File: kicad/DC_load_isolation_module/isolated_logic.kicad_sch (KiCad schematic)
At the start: 40 parts, among them Q17 MMBT5401, Q18 MMBT5401, Q2 MMBT5401, Q3 MMBT5401, Q4 MMBT5551L, Q7 MMBT5551L, U1 LTV-817S, U3 LTV-817S

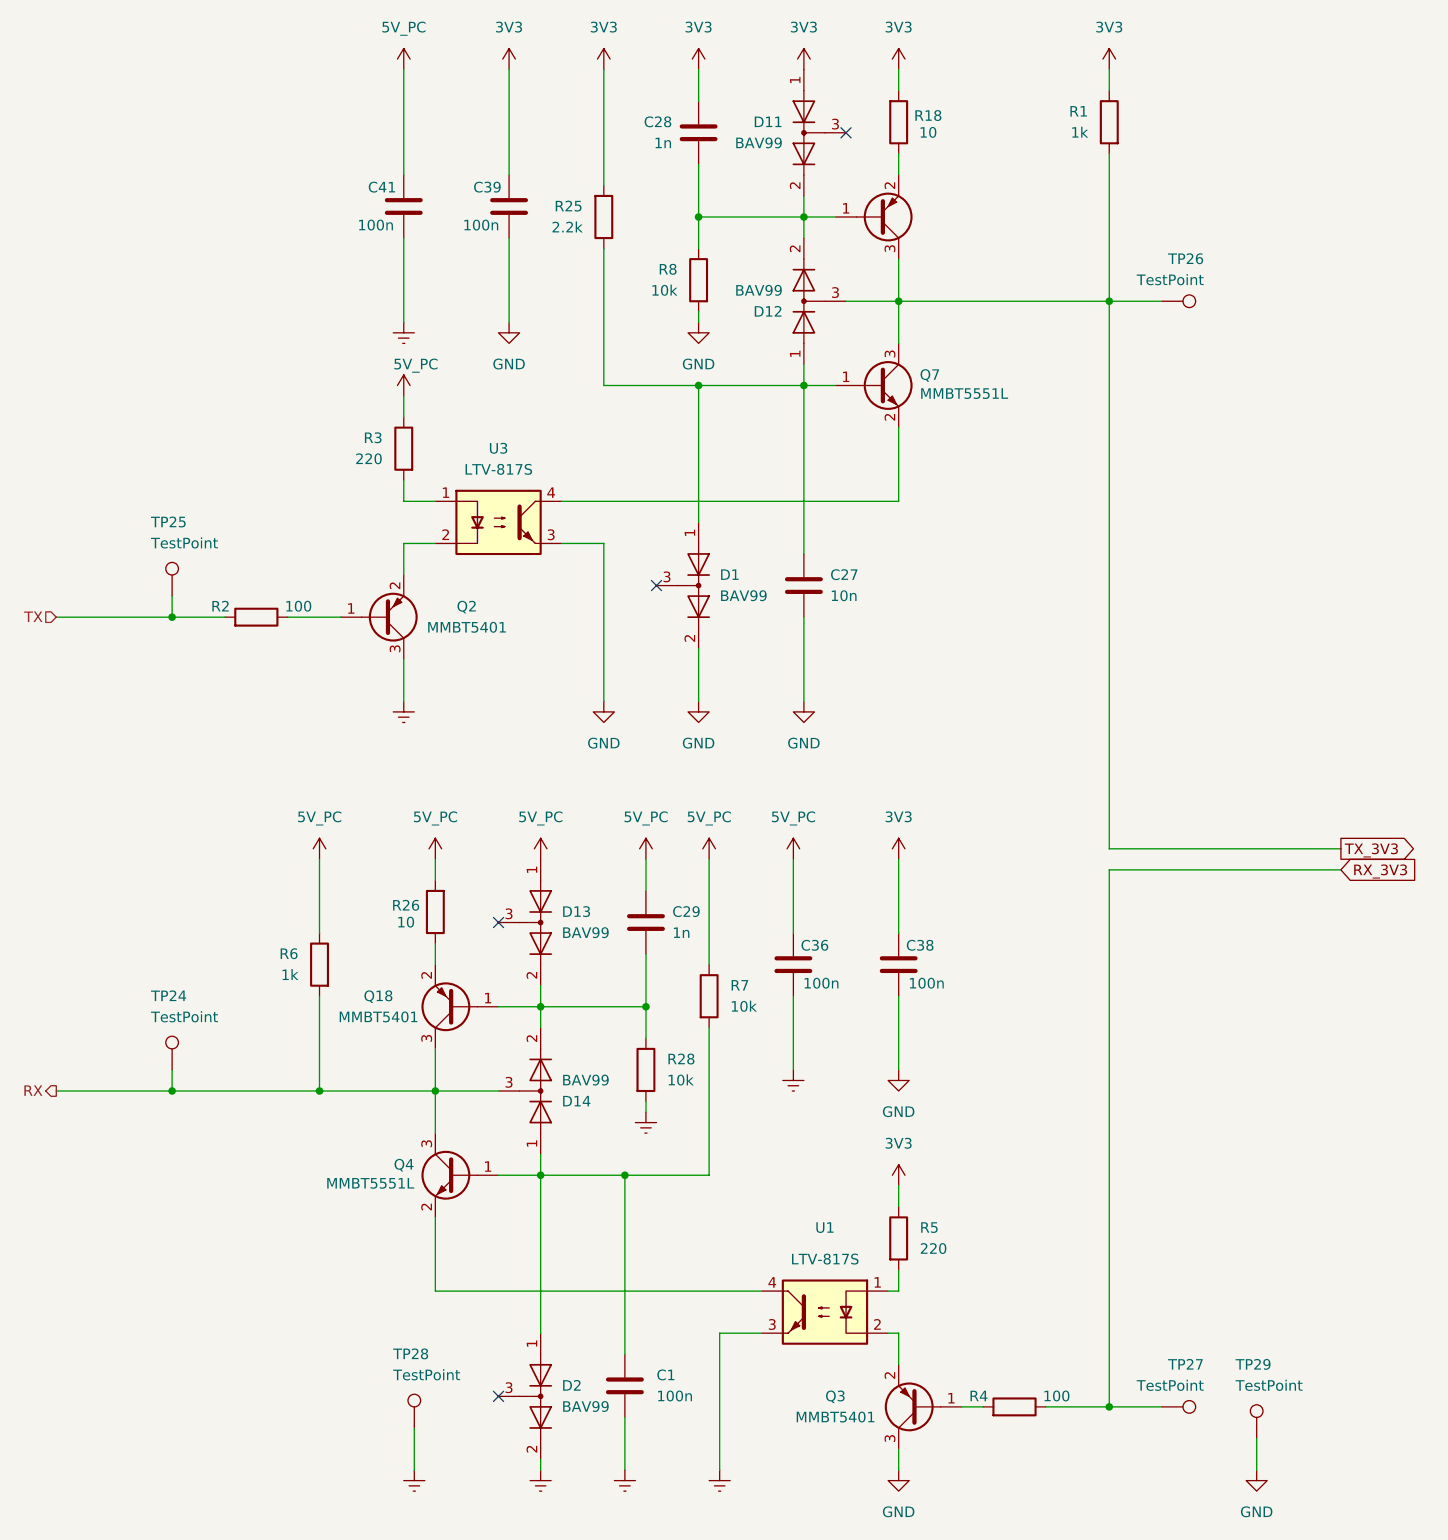
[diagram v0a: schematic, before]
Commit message: Fixes
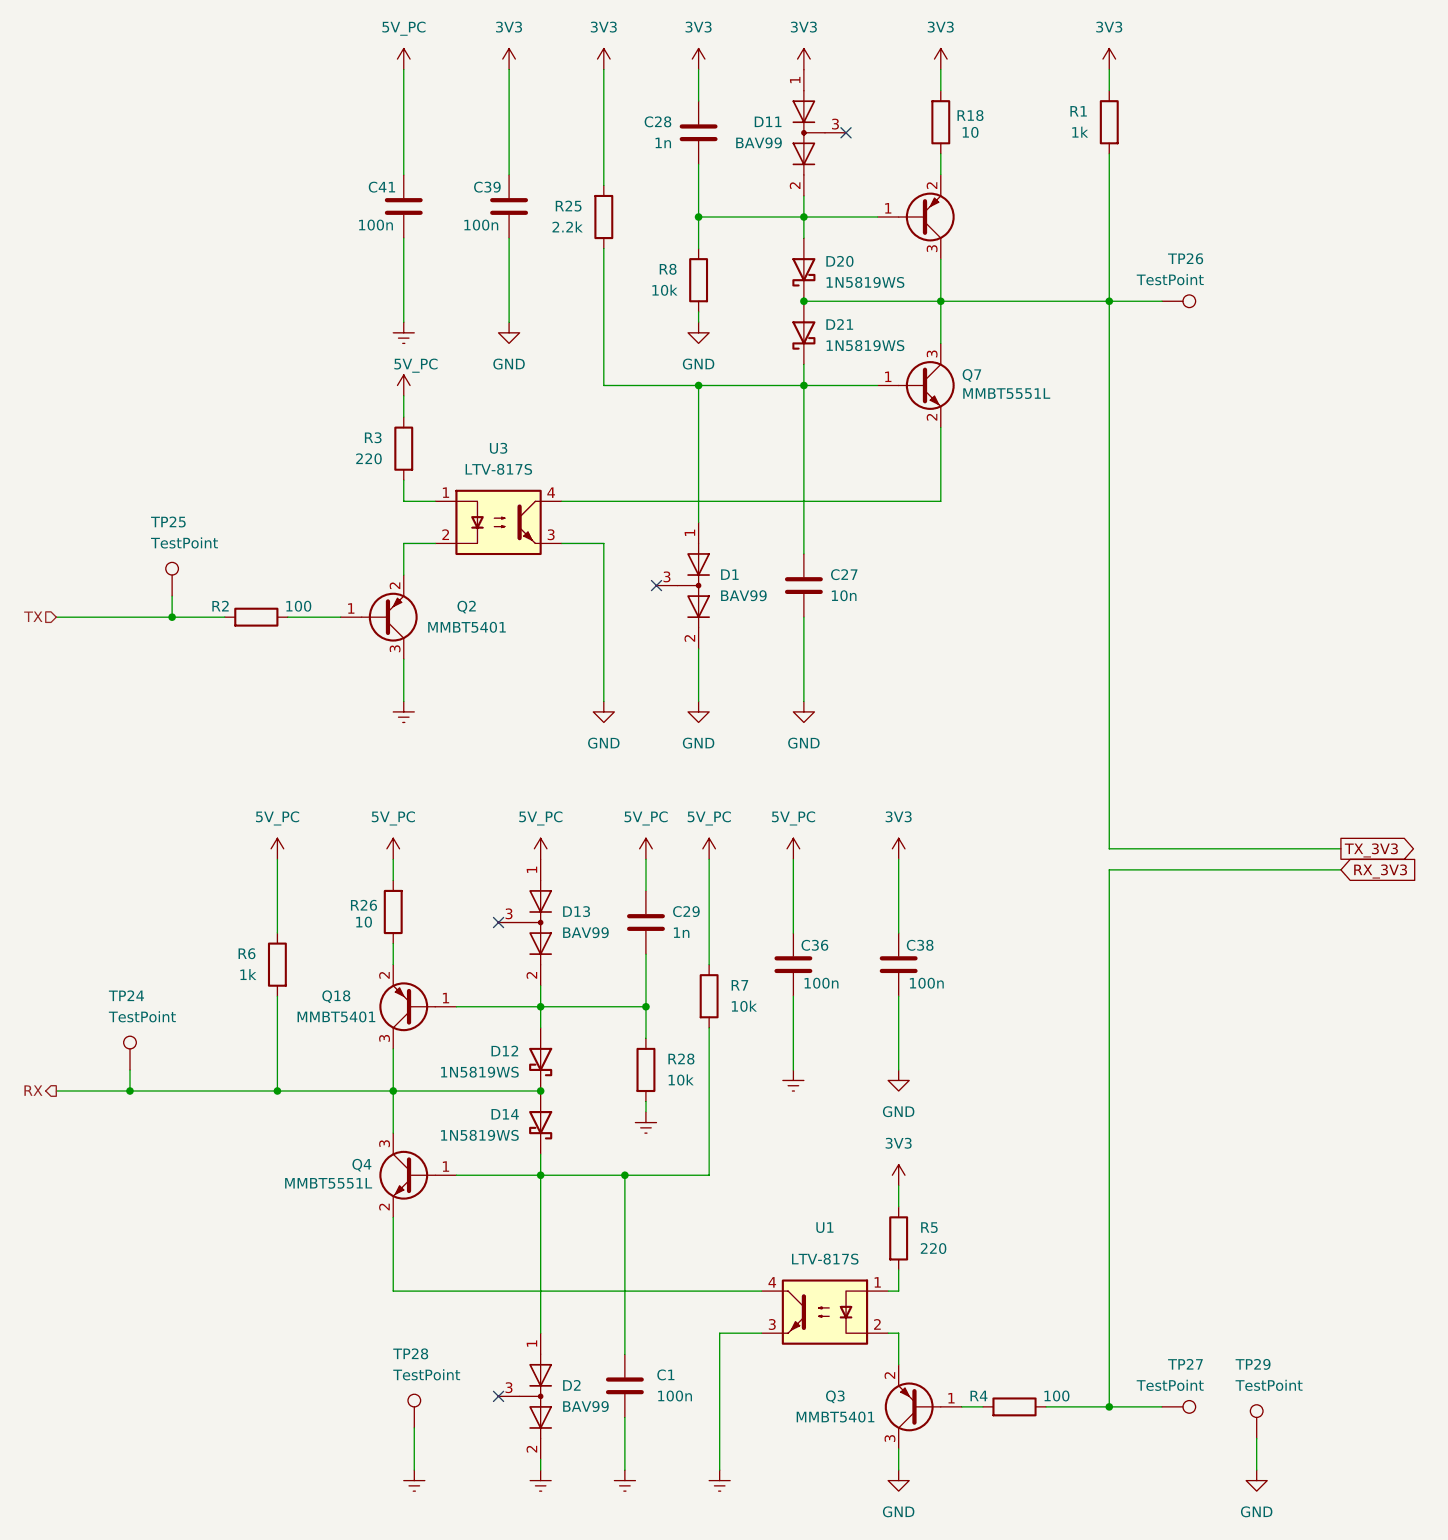
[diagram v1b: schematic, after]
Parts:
- removed D12, D14: BAV99, Package_TO_SOT_SMD:SOT-23, symbol Diode:BAV99
- added D12, D14, D20, D21: 1N5819WS, Diode_SMD:D_SOD-323, symbol Diode:1N5819WS
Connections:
- net RX: now also D12.1 (K), D14.2 (A)
- net TX_3V3: now also D20.1 (K), D21.2 (A)
- net at C29.1, D13.2 (A), Q18.1 (B)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: now also D12.2 (A)
- net at C28.1, D11.2 (A), Q17.1 (B)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: now also D20.2 (A)
- net at C27.2, D1.1 (K), Q7.1 (B)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: now also D21.1 (K)
- net at C1.2, D2.1 (K), Q4.1 (B)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: now also D14.1 (K)
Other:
- moved on the sheet: Q18, Q4, Q7, R18, R26, R6, TP24
